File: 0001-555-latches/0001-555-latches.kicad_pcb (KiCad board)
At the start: 2 copper layers, 37 parts, among them J1 DC_IN, J2 ASTBL_OUT, J3 BSTBL_OUT, J4 MSTBL_OUT, SW1 SW_Push, SW2 SW_Push, SW3 SW_Push, U1 NE555P, U2 NE555P, U3 NE555P

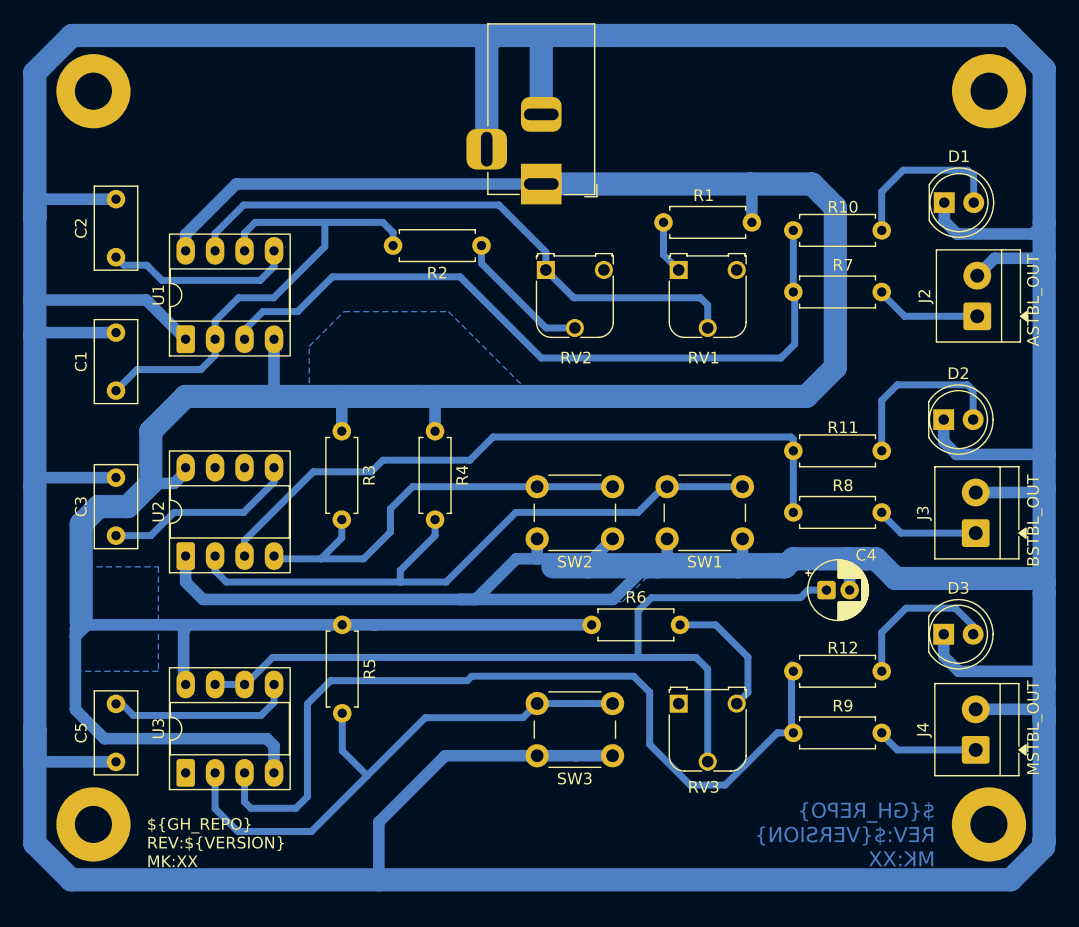
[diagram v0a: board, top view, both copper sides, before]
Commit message: Closing PCB
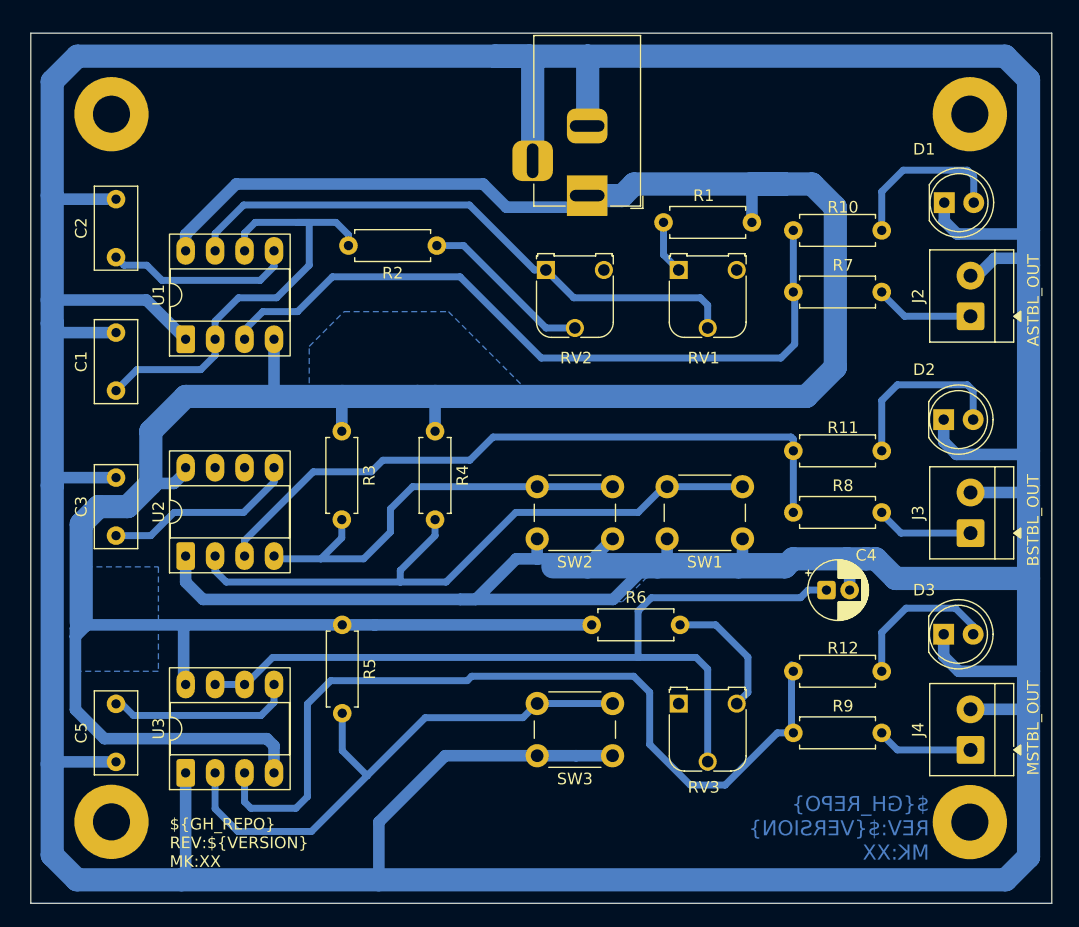
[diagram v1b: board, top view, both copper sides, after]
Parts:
- removed REF** (x4): MountingHole_3.2mm_M3_Pad, MountingHole:MountingHole_3.2mm_M3_Pad
- added MNT1: MountingHole_3.2mm_M3_Pad, MountingHole:MountingHole_3.2mm_M3_Pad, F.Cu at (108.0, 68.0)
- added MNT2: MountingHole_3.2mm_M3_Pad, MountingHole:MountingHole_3.2mm_M3_Pad, F.Cu at (181.9, 68.0)
- added MNT3: MountingHole_3.2mm_M3_Pad, MountingHole:MountingHole_3.2mm_M3_Pad, F.Cu at (181.9, 129.0)
- added MNT4: MountingHole_3.2mm_M3_Pad, MountingHole:MountingHole_3.2mm_M3_Pad, F.Cu at (108.0, 129.0)
- moved J1 4.08 mm to (149.0, 75.0)
- moved R2 3.85 mm to (136.0, 79.3)
- moved J2 0.58 mm to (182.0, 85.4)
- moved J3 0.45 mm to (182.0, 104.1)
- moved J4 0.45 mm to (182.0, 122.8)
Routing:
- net GND: track 595.0 -> 576.6 mm
- net VCC: track 251.8 -> 256.3 mm
- net Net-(U1-THR): track 43.2 -> 39.8 mm
- net Net-(R2-Pad1): track 11.9 -> 14.8 mm
- net Net-(U1-DIS): track 51.4 -> 50.5 mm
- net /ASTBL_OUT: track 9.17 -> 8.59 mm
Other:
- board outline added: 88 x 75 mm
